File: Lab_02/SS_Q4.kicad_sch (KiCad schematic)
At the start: 31 parts

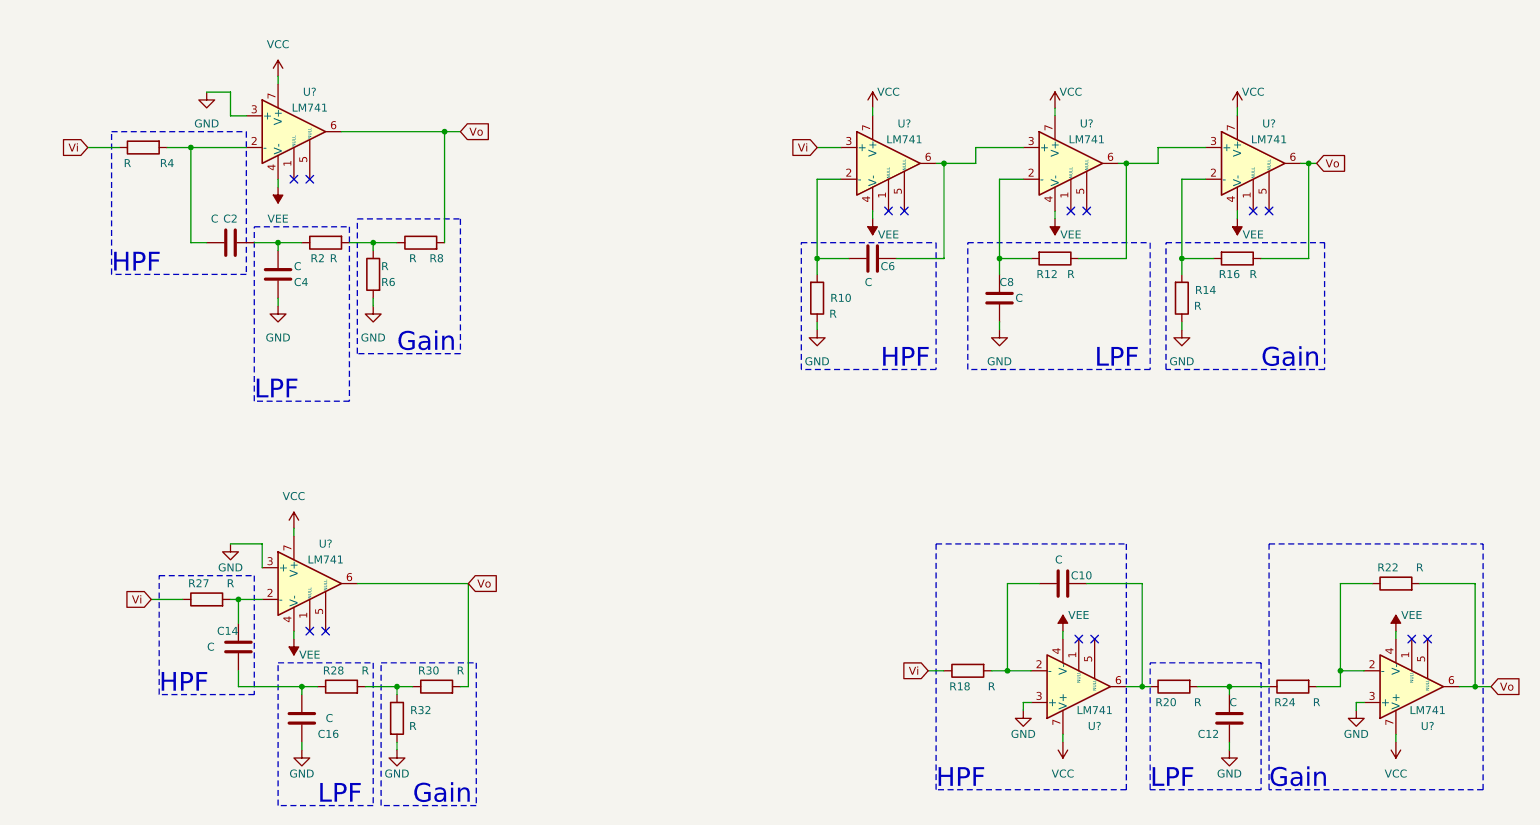
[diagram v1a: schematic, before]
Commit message: Finish Lab 02 Saturday Schematics
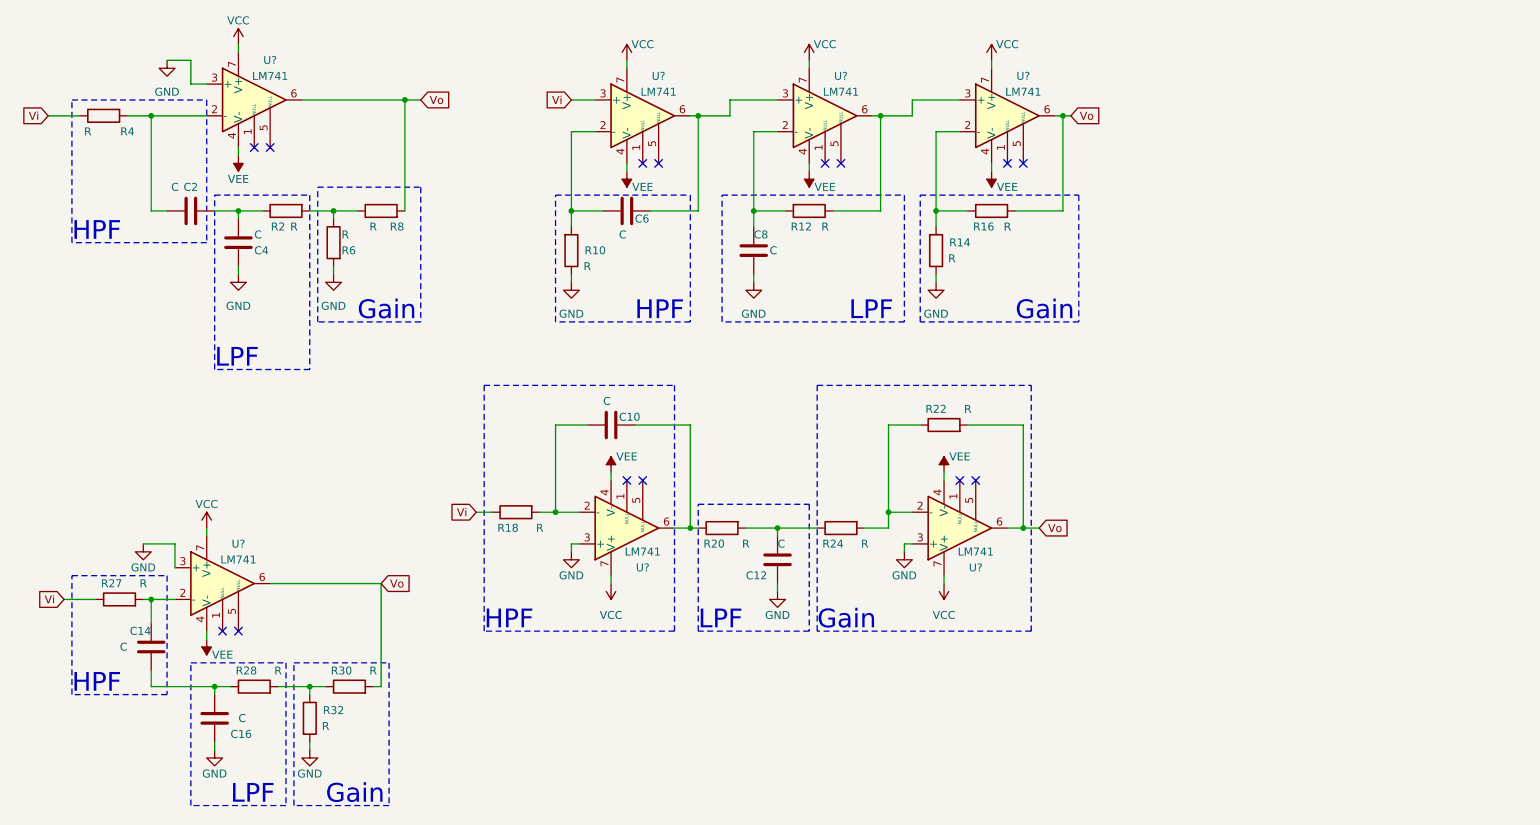
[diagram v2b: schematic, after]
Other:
- company: (none) -> Jim Horwitz & Mark Vaughn, Jork Incorporated
- title: (none) -> Active Bandpass Filter Topologies
- moved on the sheet: C10, C12, C14, C16, C2, C4, C6, C8, R10, R12, R14, R16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
